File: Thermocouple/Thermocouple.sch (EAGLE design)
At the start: 21 parts

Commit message: New versions of IntegerLabs library, RotaryEncoder, and Thermocouple
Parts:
- LED1: device adafruit:LEDCHIPLED_0805 -> adafruit:LEDCHIP-LED0805
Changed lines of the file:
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@@
 <part name="R1" library="SparkFun-Passives" deviceset="RESISTOR" device="0805-RES" value="680"/>
 <part name="U$2" library="IntegerLabs" deviceset="FOOTPRINT" device="FOOTPRINT-2" value="FOOTPRINTFOOTPRINT-2"/>
-<part name="LED1" library="adafruit" deviceset="LED" device="CHIPLED_0805"/>
+<part name="LED1" library="adafruit" deviceset="LED" device="CHIP-LED0805"/>
 <part name="R2" library="SparkFun-Resistors" deviceset="RESISTOR" device="0805-RES" value="1"/>
 <part name="U$1" library="IntegerLabs" deviceset="AD8495" device=""/>

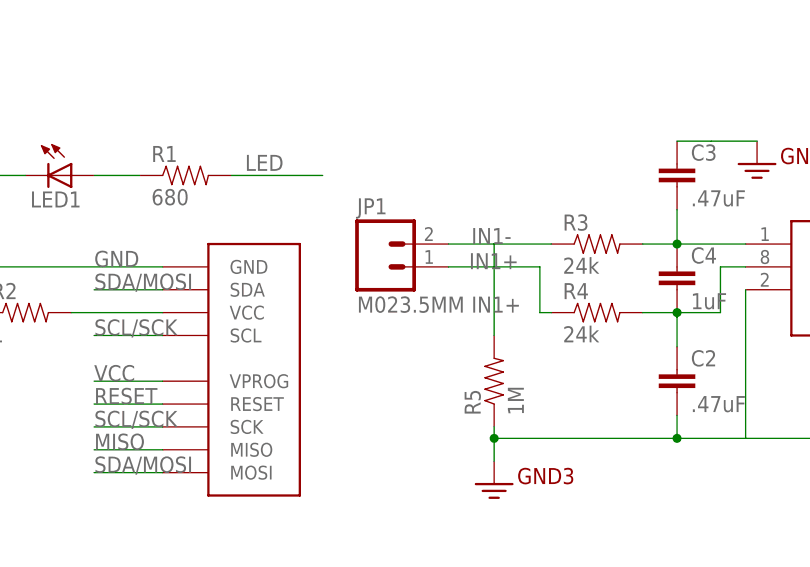
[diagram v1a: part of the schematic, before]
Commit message: Checkpointing PCB designs
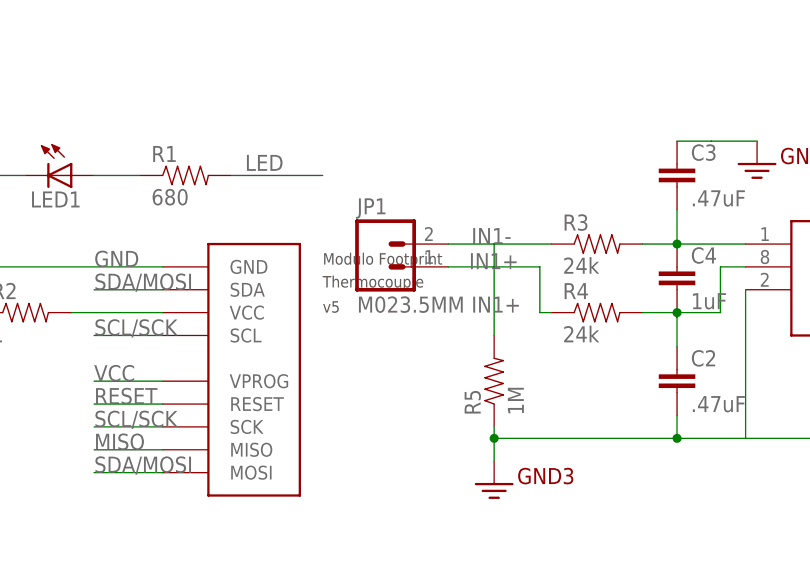
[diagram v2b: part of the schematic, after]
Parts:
- U$2: BOARD (none) -> Thermocouple; VERSION (none) -> v5
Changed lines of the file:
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@@
 <layers>
 <layer number="1" name="Top" color="4" fill="1" visible="no" active="no"/>
+<layer number="2" name="Route2" color="1" fill="3" visible="no" active="no"/>
+<layer number="3" name="Route3" color="4" fill="3" visible="no" active="no"/>
+<layer number="14" name="Route14" color="1" fill="6" visible="no" active="no"/>
+<layer number="15" name="Route15" color="4" fill="6" visible="no" active="no"/>
 <layer number="16" name="Bottom" color="1" fill="1" visible="no" active="no"/>
 <layer number="17" name="Pads" color="2" fill="1" visible="no" active="no"/>
@@
 <part name="C1" library="SparkFun-Capacitors" deviceset="CAP" device="0805" value=".47uF"/>
 <part name="R1" library="SparkFun-Passives" deviceset="RESISTOR" device="0805-RES" value="680"/>
-<part name="U$2" library="IntegerLabs" deviceset="FOOTPRINT" device="FOOTPRINT-2" value="FOOTPRINTFOOTPRINT-2"/>
+<part name="U$2" library="IntegerLabs" deviceset="FOOTPRINT" device="FOOTPRINT-2" value="FOOTPRINTFOOTPRINT-2">
+<attribute name="BOARD" value="Thermocouple"/>
+<attribute name="VERSION" value="v5"/>
+</part>
 <part name="LED1" library="adafruit" deviceset="LED" device="CHIP-LED0805"/>
 <part name="R2" library="SparkFun-Resistors" deviceset="RESISTOR" device="0805-RES" value="1"/>

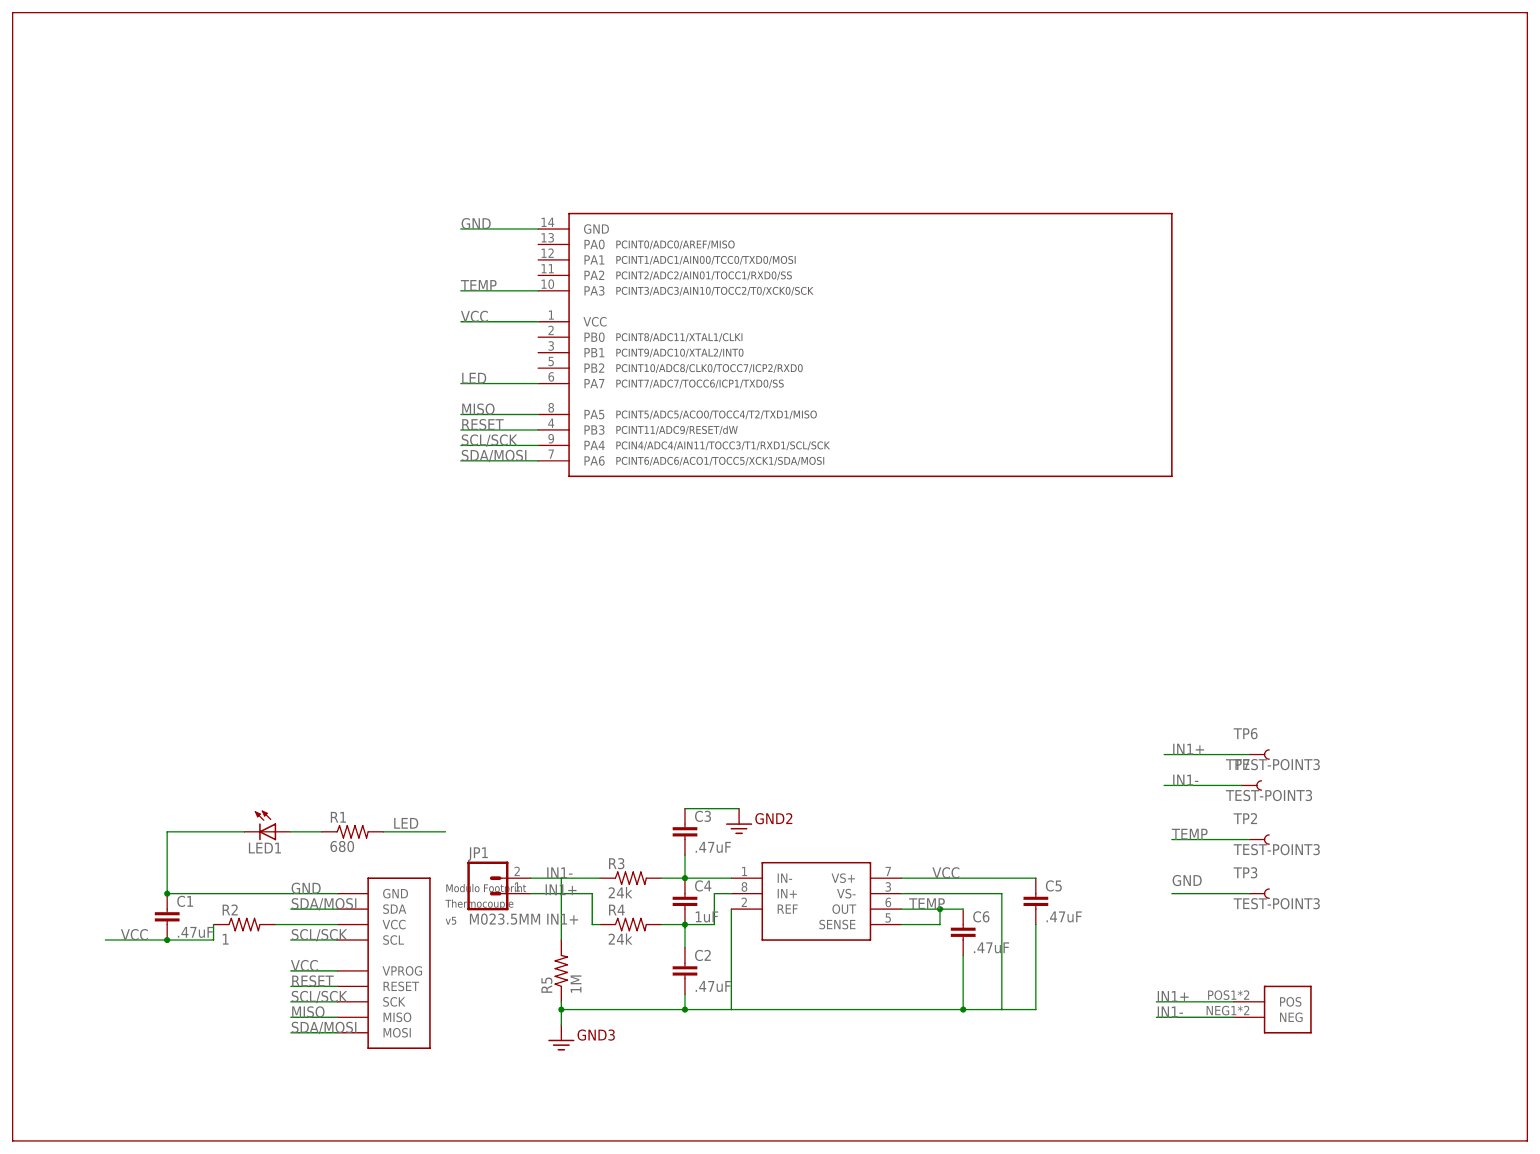
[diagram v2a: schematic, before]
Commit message: Various updates
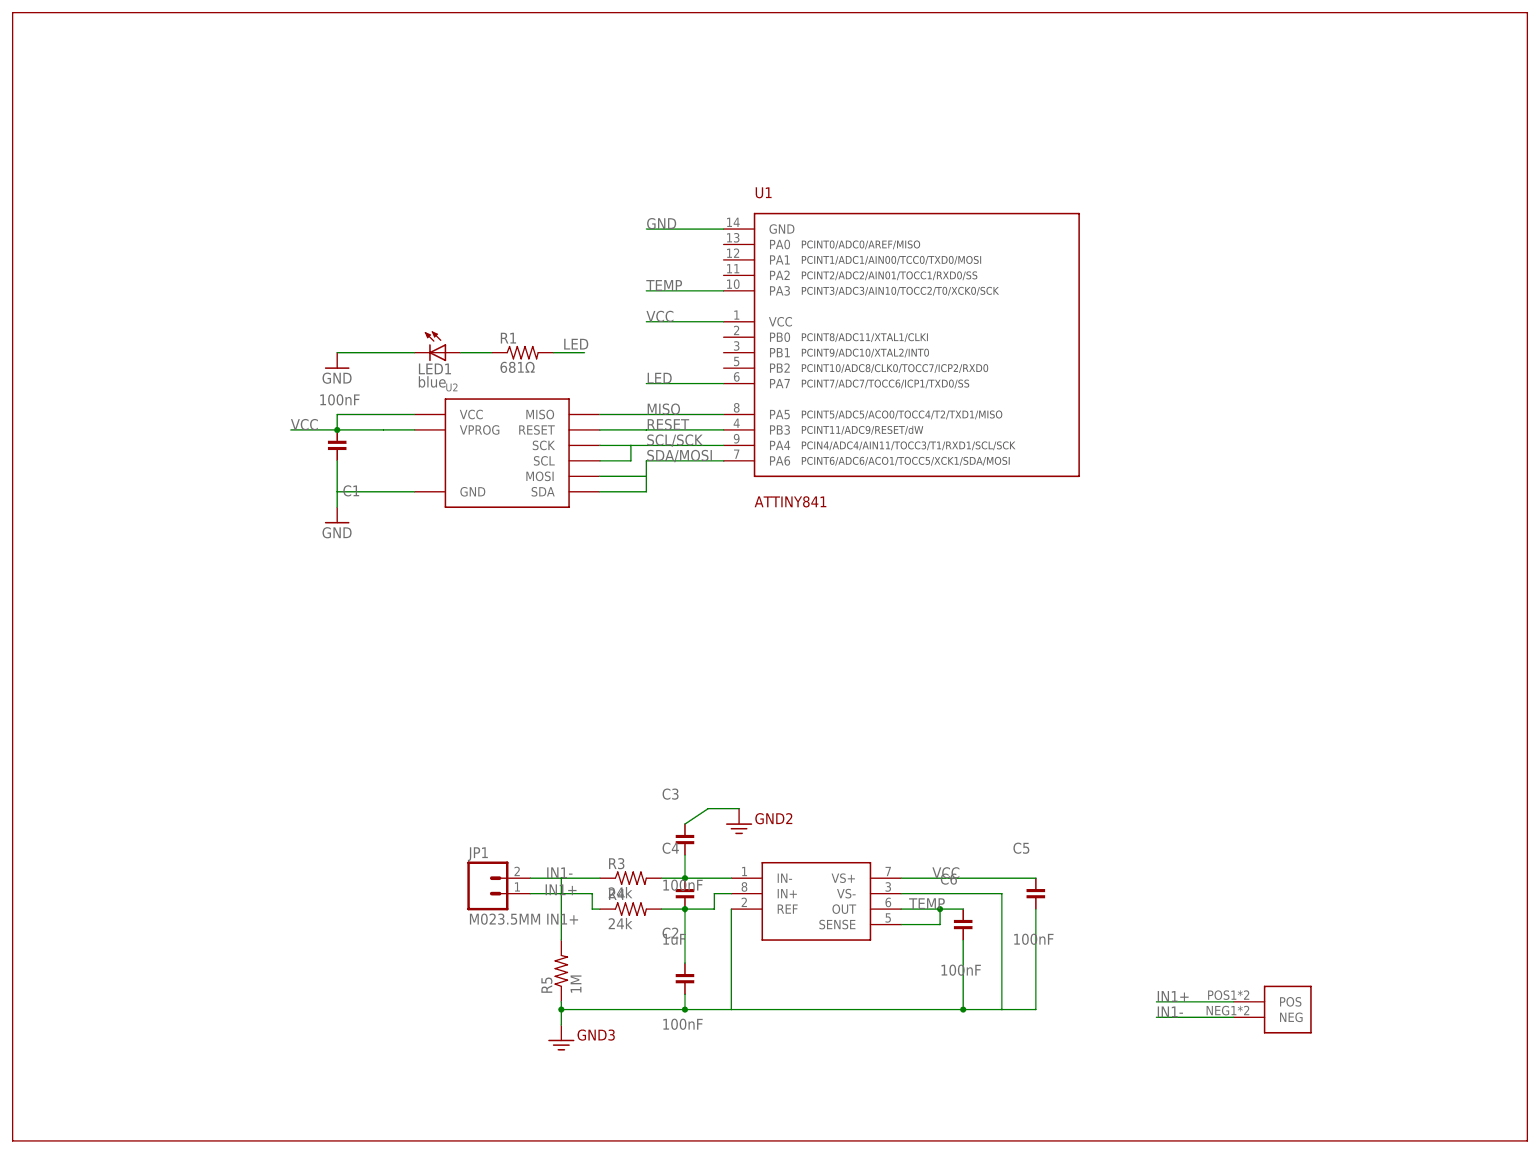
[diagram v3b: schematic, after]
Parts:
- removed R2: 1, SparkFun-Resistors:RESISTOR0805-RES
- removed TP2, TP3, TP6, TP7: TEST-POINT3, SparkFun-Passives:TEST-POINT3
- removed U$2: FOOTPRINTFOOTPRINT-2, IntegerLabs:FOOTPRINTFOOTPRINT-2
- removed U$3: TINY841, IntegerLabs:TINY841
- added U1: ATTINY841, Modulo:ATTINY841
- added U2: EXCLUDE, Modulo:DEVICE-PCB
- C1, C2, C3, C5, C6: value .47uF -> 100nF; device SparkFun-Capacitors:CAP0805 -> Modulo:CAPACITOR-100NF
- C4: device SparkFun-Capacitors:CAP0805 -> Modulo:CAPACITOR-1UF
- JP1: PARTNUM (none) -> OSTTE020104
- LED1: value (none) -> blue; device adafruit:LEDCHIP-LED0805 -> Modulo:LED-0805-BLUE
- R1: value 680 -> 681Ω; device SparkFun-Passives:RESISTOR0805-RES -> Modulo:RESISTOR-681Ω
- R3, R4: device SparkFun-Resistors:RESISTOR0805-RES -> Modulo:RESISTOR-0603; PARTNUM (none) -> ERJ-3EKF2402V
- R5: device SparkFun-Resistors:RESISTOR0805-RES -> Modulo:RESISTOR-0603; PARTNUM (none) -> ERJ-3EKF1004V
- U$1: PARTNUM (none) -> AD8495ARMZ-R7
- U$4: PARTNUM (none) -> Keystone 3572, 3549
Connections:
- removed net N$2: R2.2, U$2.VCC
- net GND: now also U1.GND, U2.GND; no longer TP3.1, U$2.GND, U$3.GND
- net IN1+: no longer TP6.1
- net IN1-: no longer TP7.1
- net LED: now also U1.PA7; no longer U$3.PA7
- net MISO: now also U1.PA5, U2.MISO; no longer U$2.MISO, U$3.PA5
- net RESET: now also U1.PB3, U2.RESET; no longer U$2.RESET, U$3.PB3
- net SCL/SCK: now also U1.PA4, U2.SCK, U2.SCL; no longer U$2.SCK, U$2.SCL, U$3.PA4
- net SDA/MOSI: now also U1.PA6, U2.MOSI, U2.SDA; no longer U$2.MOSI, U$2.SDA, U$3.PA6
- net TEMP: now also U1.PA3; no longer TP2.1, U$3.PA3
- net VCC: now also U1.VCC, U2.VCC, U2.VPROG; no longer R2.1, U$2.VPROG, U$3.VCC
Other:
- moved on the sheet: LED1, R1, R4
